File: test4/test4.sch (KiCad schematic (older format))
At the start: 2 parts, among them U1 74LS245, U2 74LS245

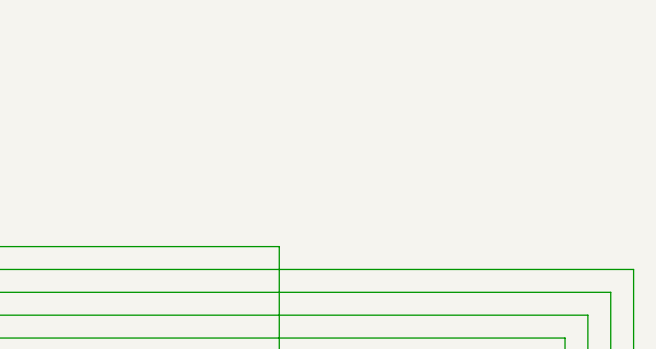
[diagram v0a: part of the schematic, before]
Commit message: playing with schematic symbol editor
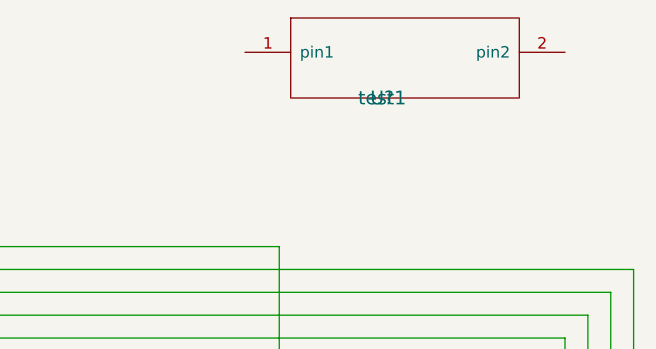
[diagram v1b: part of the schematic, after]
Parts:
- added U?: test1, symbol test1
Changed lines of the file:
@@
 LIBS:contrib
 LIBS:valves
+LIBS:test1
+LIBS:test4-cache
 EELAYER 25 0
 EELAYER END
@@
 	4950 5050 4950 4850
 Connection ~ 4950 4850
+$Comp
+L test1 U?
+U 1 1 5672C530
+P 7400 1600
+F 0 "U?" H 7400 1600 60  0000 C CNN
+F 1 "test1" H 7400 1600 60  0000 C CNN
+F 2 "" H 7400 1600 60  0000 C CNN
+F 3 "" H 7400 1600 60  0000 C CNN
+	1    7400 1600
+	1    0    0    -1
+$EndComp
 $EndSCHEMATC
